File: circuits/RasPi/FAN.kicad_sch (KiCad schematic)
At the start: 5 parts, among them J13 Conn_01x03_MountingPin, Q25 BSS138, Q26 SSM3J332R

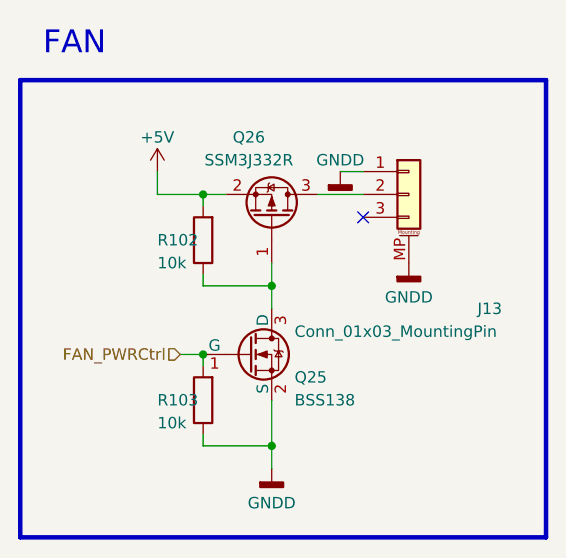
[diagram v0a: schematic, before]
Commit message: 更新
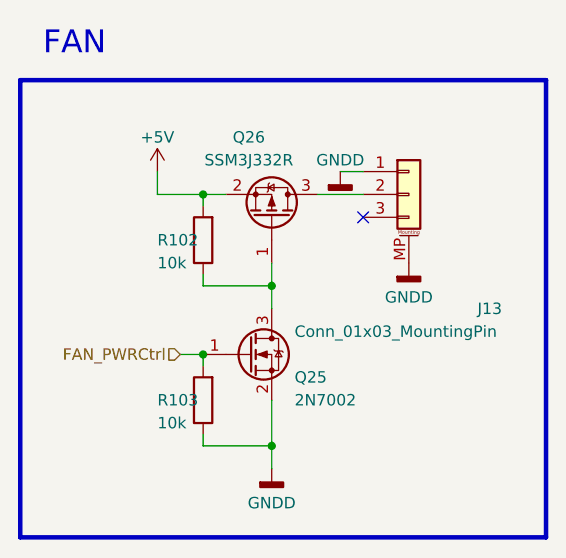
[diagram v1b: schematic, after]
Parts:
- removed Q25: BSS138, Package_TO_SOT_SMD:SOT-23, symbol Device:Q_NMOS_GSD
- added Q25: 2N7002, Package_TO_SOT_SMD:SOT-23, symbol Transistor_FET:2N7002
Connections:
- net FAN_PWRCtrl: now also Q25.1 (G)
- net GNDD: now also Q25.2 (S)
- net at Q26.1 (G), R102.1: now also Q25.3 (D)
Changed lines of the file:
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@@
   (junction (at 142.24 99.06) (diameter 0) (color 0 0 0 0)
   )
+  (junction (at 134.62 88.9) (diameter 0) (color 0 0 0 0)
+  )
   (junction (at 134.62 71.12) (diameter 0) (color 0 0 0 0)
-  )
-  (junction (at 134.62 88.9) (diameter 0) (color 0 0 0 0)
   )
   (junction (at 142.24 81.28) (diameter 0) (color 0 0 0 0)
@@
     )
   )
+  (symbol (lib_id "Transistor_FET:2N7002") (at 139.7 88.9 0) (unit 1)
+    (in_bom yes) (on_board yes) (dnp no)
+    (property "Reference" "Q25" (at 144.78 91.44 0)
+      (effects (font (size 1.27 1.27)) (justify left))
+    )
+    (property "Value" "2N7002" (at 144.78 93.98 0)
+      (effects (font (size 1.27 1.27)) (justify left))
+    )
+    (property "Footprint" "Package_TO_SOT_SMD:SOT-23" (at 144.78 90.805 0)
+      (effects (font (size 1.27 1.27) italic) (justify left) hide)
+    )
+    (property "Datasheet" "https://www.onsemi.com/pub/Collateral/NDS7002A-D.PDF" (at 144.78 92.71 0)
+      (effects (font (size 1.27 1.27)) (justify left) hide)
+    )
+    (pin "3")
+    (pin "1")
+    (pin "2")
+    (instances
+      (project "RasPi"
+        (path "/689a9e74-f202-4ea4-bfbb-4341f2549250/fddad0c3-2af8-46e3-8794-fa1122d24d51/ffa9c1a5-d3a0-4e0c-a61b-1846c86fcc40"
+          (reference "Q25") (unit 1)
+        )
+      )
+    )
+  )
   (symbol (lib_id "power:GNDD") (at 157.48 78.74 0) (unit 1)
     (in_bom yes) (on_board yes) (dnp no)
@@
         )
       )
-    )
-  )
-  (symbol (lib_name "Q_NMOS_GSD_1") (lib_id "Device:Q_NMOS_GSD") (at 139.7 88.9 0) (unit 1)
-    (in_bom yes) (on_board yes) (dnp no)
-    (property "Reference" "Q25" (at 144.78 91.44 0)
-      (effects (font (size 1.27 1.27)) (justify left))
-    )
-    (property "Value" "BSS138" (at 144.78 93.98 0)
-      (effects (font (size 1.27 1.27)) (justify left))
-    )
-    (property "Footprint" "Package_TO_SOT_SMD:SOT-23" (at 144.78 86.36 0)
-      (effects (font (size 1.27 1.27)) hide)
-    )
-    (property "Datasheet" "~" (at 139.7 88.9 0)
-      (effects (font (size 1.27 1.27)) hide)
-    )
-    (pin "1")
-    (pin "2")
-    (pin "3")
-    (instances
-      (project "RasPi"
-        (path "/689a9e74-f202-4ea4-bfbb-4341f2549250/fddad0c3-2af8-46e3-8794-fa1122d24d51/ffa9c1a5-d3a0-4e0c-a61b-1846c86fcc40"
-          (reference "Q25") (unit 1)
-        )
-      )
